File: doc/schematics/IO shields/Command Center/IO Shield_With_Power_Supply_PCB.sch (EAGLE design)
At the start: 41 parts, among them IC1 74S08D, IC2 74LS04D, IC3 74S08D, IC4 74LS32D, J1 POW_CONNECTFEMALE-RA, J2 POW_CONNECTFEMALE-RA, J3 POW_CONNECTFEMALE-RA, J4 POW_CONNECTFEMALE-RA, J5 POW_CONNECTFEMALE-RA

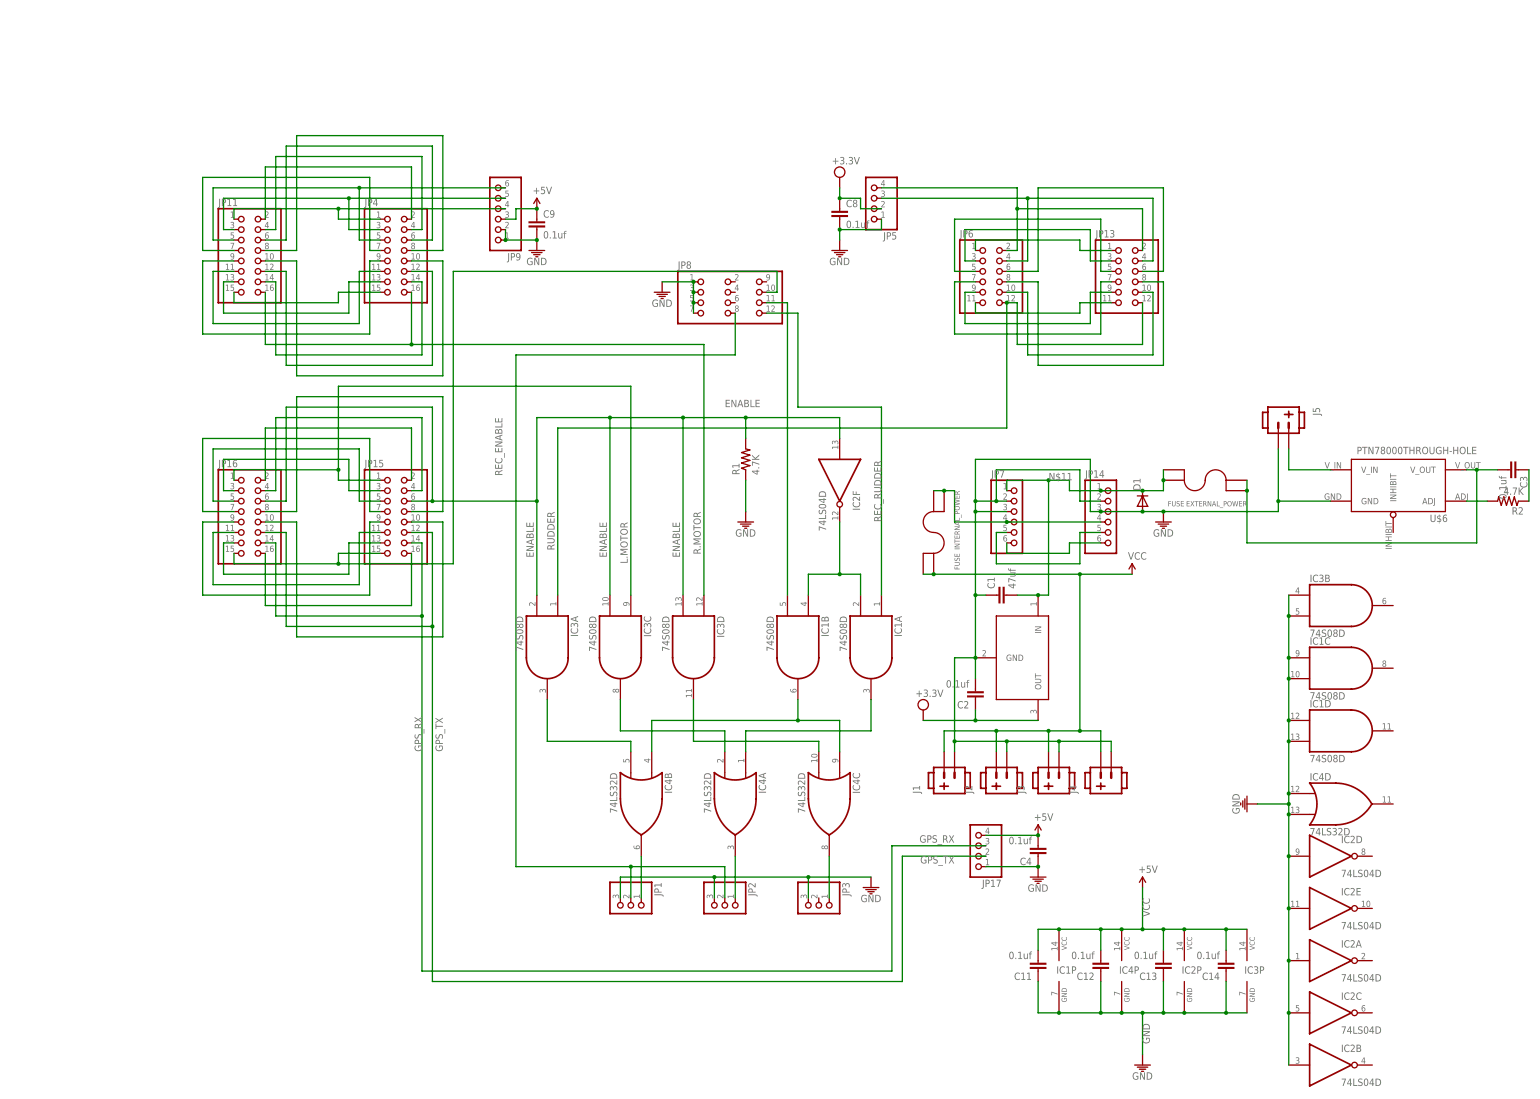
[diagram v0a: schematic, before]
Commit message: Merged in Johns physical design changes.
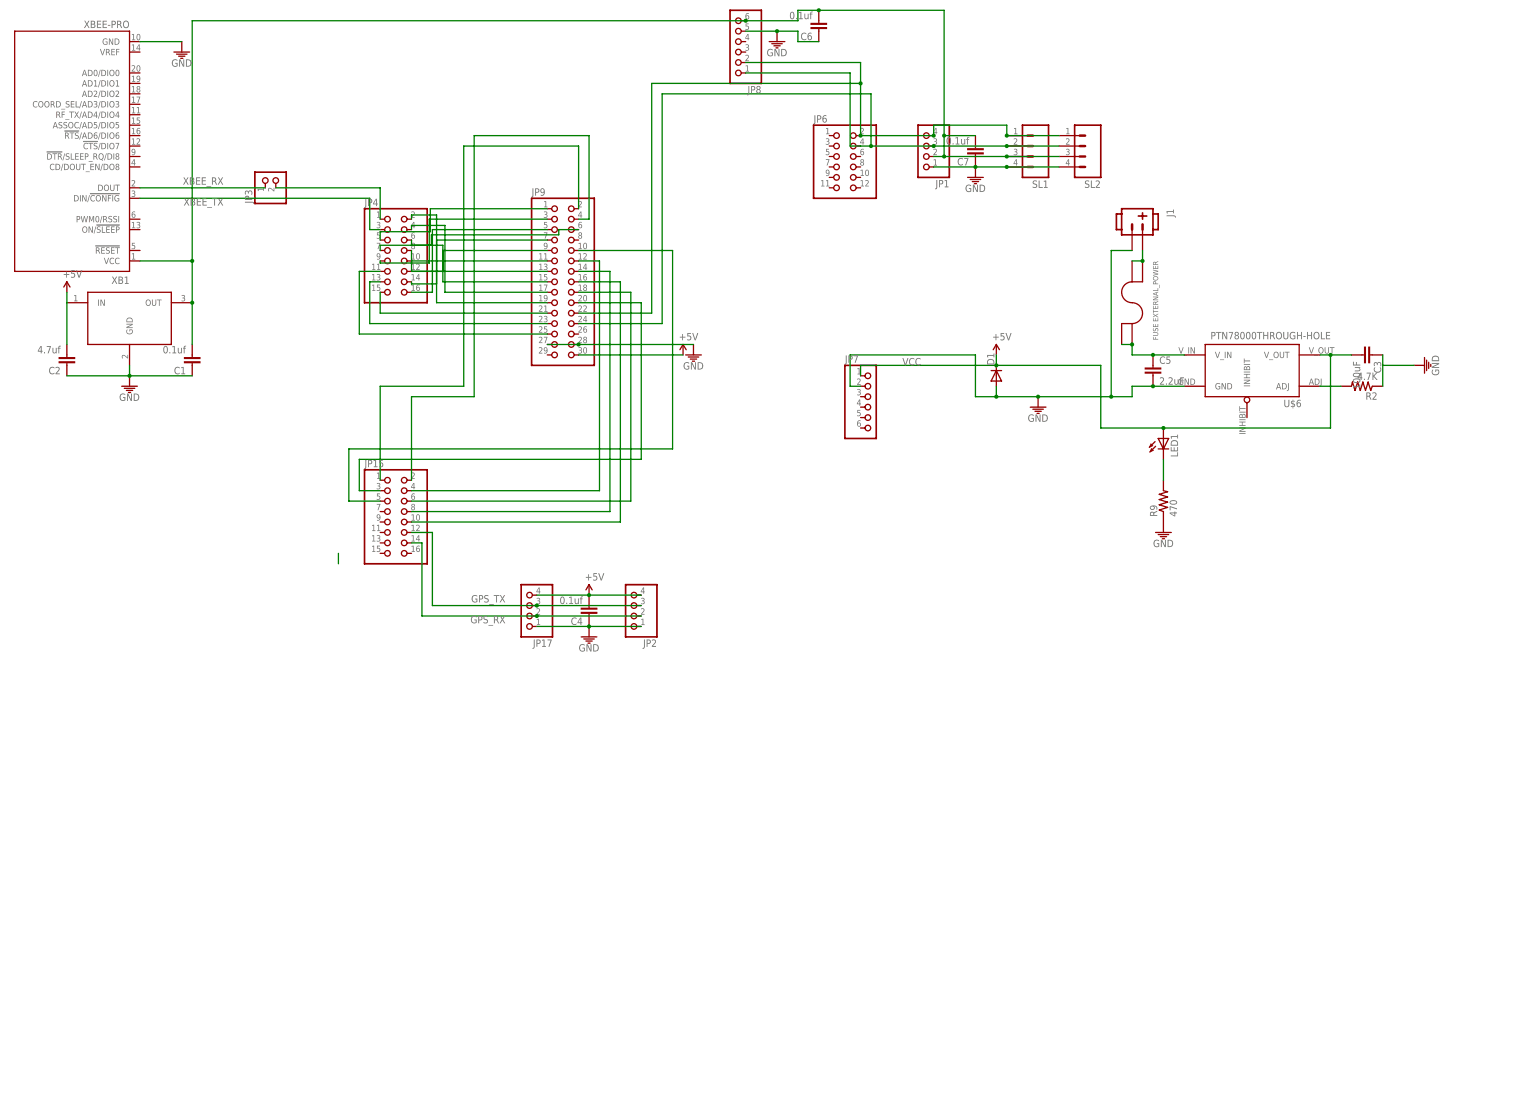
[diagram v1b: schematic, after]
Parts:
- removed C11, C12, C13, C14, C8, C9: 0.1uf, resistor:C-EUC0805
- removed IC1, IC3: 74S08D, 74xx-us:74S08D
- removed IC2: 74LS04D, 74xx-us:74LS04D
- removed IC4: 74LS32D, 74xx-us:74LS32D
- removed INTERNAL_POWER: FUSE, ASL:FUSE
- removed J2, J3, J4, J5: POW_CONNECTFEMALE-RA, ASL:POW_CONNECTFEMALE-RA
- removed JP11, JP16: (no value), pinhead:PINHD-2X8
- removed JP13: (no value), pinhead:PINHD-2X6
- removed JP14: (no value), pinhead:PINHD-1X6
- removed JP5: (no value), SDLogger:PINHD-1X4
- removed R1: 4.7K, ASL:RESISTOR0805-RES
- removed U$1: LM3940IMP-3.3, LM3940:LM3940IMP-3.3
- added C5: 2.2uF, resistor:C-EUC0805
- added C6, C7: 0.1uf, resistor:C-EUC0805
- added LED1: (no value), ASL:LED-FKIT-1206
- added R9: 470, ASL:RESISTOR0805-RES
- added SL1, SL2: (no value), ASL:M04LOCK
- added U$7: LM3940IMP-3.3, LM3940:LM3940IMP-3.3
- added XB1: XBEE-PRO, maxstream:XBEE-PRO
- C1: value 47uf -> 0.1uf
- C2: value 0.1uf -> 4.7uf
- C3: value 0.1uf -> 100uF
- J1: value POW_CONNECTFEMALE-RA -> POW_CONNECTMALE; device ASL:POW_CONNECTFEMALE-RA -> ASL:POW_CONNECTMALE
- JP1: device pinhead:PINHD-1X3/90 -> pinhead_non_standard:PINHD-1X4
- JP2: device pinhead:PINHD-1X3/90 -> pinhead:PINHD-1X4/90
- JP3: device pinhead:PINHD-1X3/90 -> pinhead:PINHD-1X2
- JP8: device pinhead:PINHD-2X4 -> baro:PINHD-1X6
- JP9: device SDLogger:PINHD-1X6 -> pinhead:PINHD-2X15/90
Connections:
- removed net ENABLE: IC2F.I, IC3A.I1, IC3C.I1, IC3D.I1, JP15.6, JP16.6, R1.2
- removed net L.MOTOR: IC3C.I0, JP15.1, JP16.1
- removed net N$14: JP15.15, JP16.15, JP8.9
- removed net N$29: JP11.12, JP4.12
- removed net N$30: JP11.10, JP4.10
- removed net N$32: JP15.3, JP16.3
- removed net N$33: JP15.5, JP16.5
- removed net N$34: JP15.7, JP16.7
- removed net N$37: JP15.11, JP16.11
- removed net N$38: JP15.9, JP16.9
- removed net N$39: JP15.2, JP16.2
- removed net N$40: JP15.4, JP16.4
- removed net N$41: JP13.5, JP6.5
- removed net N$42: JP15.8, JP16.8
- removed net N$43: C3.1, R2.1
- removed net N$44: INTERNAL_POWER.1, INTERNAL_POWER.2, JP14.4, JP7.4
- removed net N$45: JP15.10, JP16.10
- removed net N$46: JP13.7, JP6.7
- removed net N$47: JP13.9, JP6.9
- removed net N$48: JP13.11, JP6.11
- removed net N$49: JP13.2, JP5.4, JP6.2
- removed net N$50: JP13.4, JP5.3, JP6.4
- removed net N$51: JP13.6, JP6.6
- removed net N$52: JP13.8, JP6.8
- removed net N$53: JP13.10, JP6.10
- removed net N$58: JP14.5, JP7.5
- removed net N$59: JP14.6, JP7.6
- removed net R.MOTOR: IC3D.I0, JP11.16, JP4.16
- removed net REC.MOTOR: IC1B.I1, JP8.11
- removed net REC_ENABLE: JP15.16, JP16.16
- removed net REC_RUDDER: IC1A.I0, JP8.12
- removed net RUDDER: IC3A.I0, JP13.12, JP6.12
- removed net VDD: C2.1, C8.1, JP5.2, U$1.OUT
- new net XBEE_RX: JP3.2, JP4.1
- new net XBEE_TX: JP4.3, XB1.DIN/!CONFIG
- net GND: now also C2.1, C3.1, C5.2, C6.1, C7.1, JP1.1, JP2.1, JP9.27, JP9.28, R2.1, R9.1, SL1.4, SL2.4, U$7.GND, XB1.GND; no longer C11.1, C12.1, C13.1, C14.1, C2.2, C8.2, C9.2, IC1C.I0, IC1C.I1, IC1D.I0, IC1D.I1, IC1P.GND, IC2A.I, IC2B.I, IC2C.I, IC2D.I, IC2E.I, IC2P.GND, IC3B.I0, IC3B.I1, IC3P.GND, IC4D.I0, IC4D.I1, IC4P.GND, J2.2, J3.2, J4.2, J5.2, JP1.3, JP14.2, JP14.3, JP2.3, JP3.3, JP5.1, JP7.3, JP8.1, JP8.3, JP8.7, JP9.1, JP9.2, R1.1, U$1.GND
- net GPS_RX: now also JP17.2, JP2.2; no longer JP16.14, JP17.3
- net GPS_TX: now also JP17.3, JP2.3; no longer JP16.12, JP17.2
- net N$1: now also JP3.1, XB1.DOUT; no longer IC1A.O, IC4A.I0
- net N$10: now also JP4.12, JP9.9; no longer IC4C.O, JP3.1
- net N$11: now also JP15.5, JP9.10; no longer C1.2, D1.C, EXTERNAL_POWER.3, EXTERNAL_POWER.4, JP14.1, JP7.1, U$1.IN
- net N$12: now also JP4.10, JP9.11; no longer JP1.2, JP2.2, JP8.8
- net N$13: now also C1.2, C6.2, C7.2, JP1.2, JP8.6, SL1.3, SL2.3, U$7.OUT, XB1.VCC; no longer C3.2, EXTERNAL_POWER.1, EXTERNAL_POWER.2, U$6.V_OUT
- net N$15: now also JP4.8, JP9.13; no longer JP13.1, JP6.1
- net N$16: now also C5.1, EXTERNAL_POWER.3, EXTERNAL_POWER.4; no longer J5.1
- net N$17: now also JP4.6, JP9.15; no longer JP11.3, JP4.3, JP9.5
- net N$18: now also JP4.4, JP9.17; no longer JP11.5, JP4.5, JP9.6
- net N$19: now also JP4.2, JP9.19; no longer JP11.7, JP4.7
- net N$2: now also JP4.5, JP9.1; no longer IC1B.O, IC4B.I0, IC4C.I0
- net N$20: now also JP9.21; no longer JP11.15
- net N$21: now also JP9.23; no longer JP11.13
- net N$22: now also JP9.25; no longer JP11.11
- net N$23: now also JP15.8, JP9.14; no longer JP11.9, JP4.9
- net N$24: now also JP15.6, JP9.18; no longer JP11.2, JP4.2
- net N$25: now also LED1.C, R9.2; no longer JP11.4, JP4.4
- net N$26: now also JP1.4, JP6.2, JP8.2, JP9.22, SL1.1, SL2.1; no longer JP11.6, JP4.6
- net N$27: now also JP15.10, JP9.16; no longer JP11.8, JP4.8
- net N$28: now also JP15.4, JP9.12; no longer JP11.14, JP4.14
- net N$3: now also EXTERNAL_POWER.1, EXTERNAL_POWER.2, J1.1; no longer IC1A.I1, IC1B.I0, IC2F.O
- net N$31: now also JP15.3, JP9.20; no longer JP13.3, JP6.3
- net N$36: now also JP1.3, JP6.4, JP8.1, JP9.24, SL1.2, SL2.2; no longer JP15.13, JP16.13
- net N$4: now also JP4.9, JP9.3; no longer JP11.1, JP4.1, JP9.4
- net N$5: now also JP4.7, JP9.6; no longer IC3D.O, IC4C.I1
- net N$6: now also JP15.1, JP9.2; no longer IC3C.O, IC4A.I1
- net N$7: now also JP15.2, JP9.4; no longer IC3A.O, IC4B.I1
- net N$8: now also JP4.16, JP9.5; no longer IC4B.O, JP1.1
- net N$9: now also JP4.14, JP9.7; no longer IC4A.O, JP2.1
- net VCC: now also C2.2, C3.2, D1.C, JP2.4, JP7.1, JP9.30, LED1.A, U$6.V_OUT, U$7.IN; no longer C11.2, C12.2, C13.2, C14.2, C9.1, IC1P.VCC, IC2P.VCC, IC3P.VCC, IC4P.VCC, INTERNAL_POWER.3, INTERNAL_POWER.4, J1.1, J2.1, J3.1, J4.1, JP9.3
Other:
- moved on the sheet: C1, C2, C3, C4, D1, EXTERNAL_POWER, J1, JP17, JP6, JP7, R2, U$6
